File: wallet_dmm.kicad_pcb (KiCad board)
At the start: 2 copper layers, 86 x 53 mm, 26 parts, among them J1 Conn_01x04, J2 Conn_01x02, Q1 T2N7002BK_LM, Q2 T2N7002BK_LM, SW1 RESET_BUTTON, SW2 BUTTON0, SW3 BUTTON1, SW4 BUTTON2, U1 STM32L051K8Tx, U2 TLC555xD, U3 MCP9700-E/TO

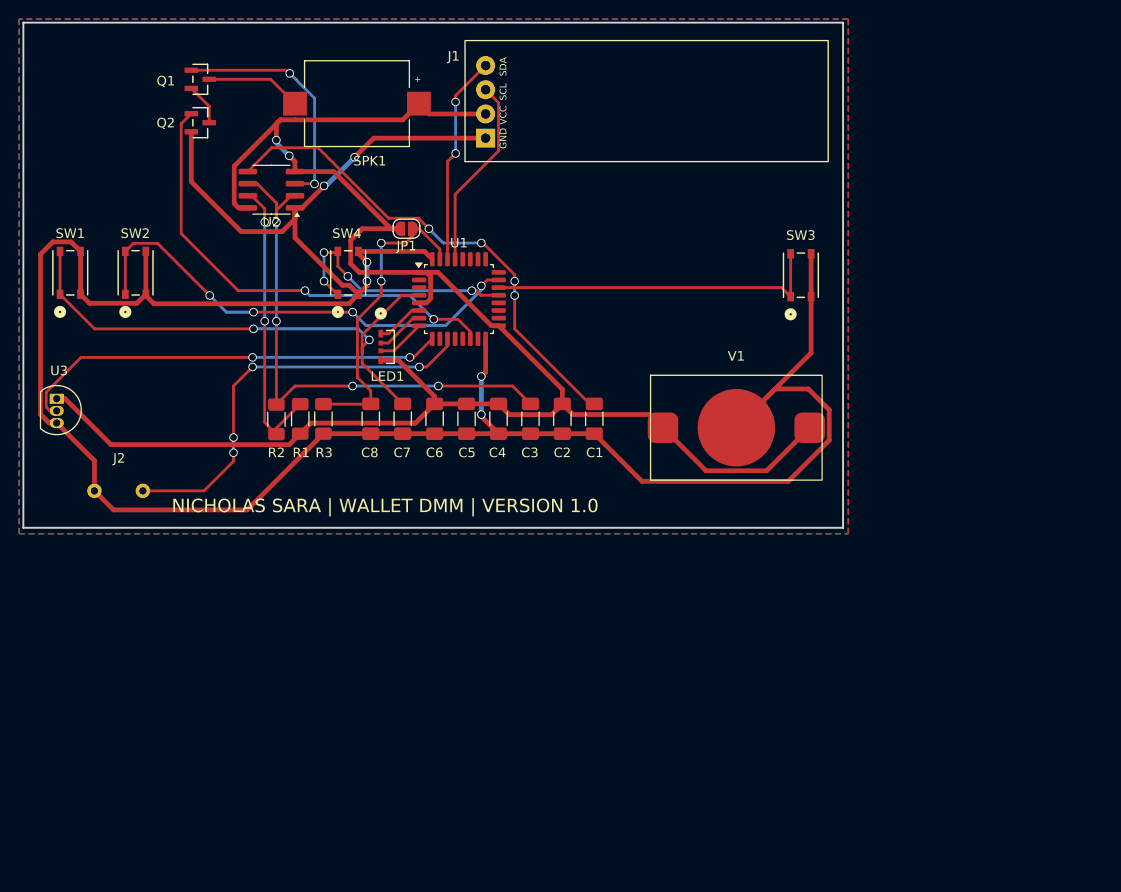
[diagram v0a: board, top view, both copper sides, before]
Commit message: Revision 2
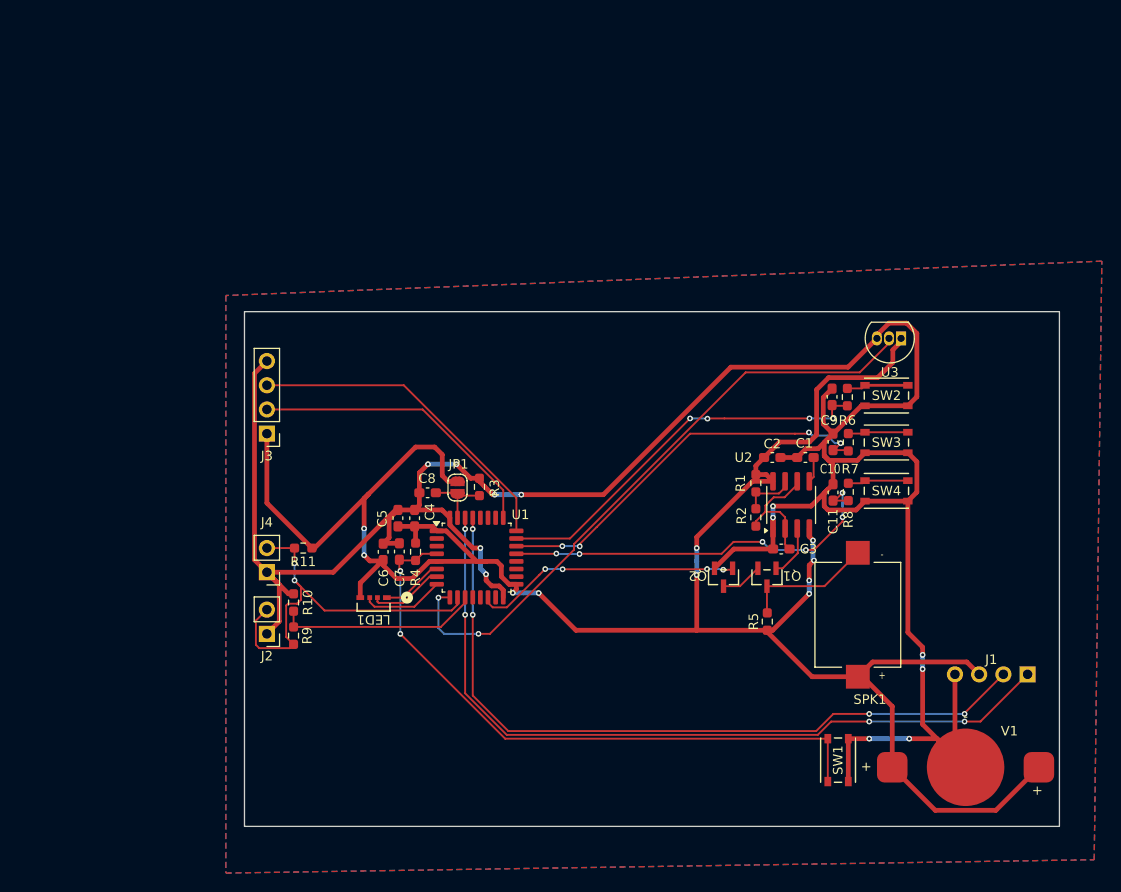
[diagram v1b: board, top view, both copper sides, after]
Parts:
- added C10: 100nF, Capacitor_SMD:C_0603_1608Metric_Pad1.08x0.95mm_HandSolder, F.Cu at (155.4, 72.9)
- added C11: 100nF, Capacitor_SMD:C_0603_1608Metric_Pad1.08x0.95mm_HandSolder, F.Cu at (155.4, 78.2)
- added C9: 100nF, Capacitor_SMD:C_0603_1608Metric_Pad1.08x0.95mm_HandSolder, F.Cu at (155.3, 68.1)
- added J3: Conn_01x04, Connector_PinHeader_2.54mm:PinHeader_1x04_P2.54mm_Vertical, F.Cu at (96.0, 72.0)
- added J4: Voltmeter, Connector_PinHeader_2.54mm:PinHeader_1x02_P2.54mm_Vertical, F.Cu at (96.0, 86.5)
- added R10: 1M, Resistor_SMD:R_0603_1608Metric_Pad0.98x0.95mm_HandSolder, F.Cu at (98.8, 89.7)
- added R11: 1M, Resistor_SMD:R_0603_1608Metric_Pad0.98x0.95mm_HandSolder, F.Cu at (99.8, 84.0)
- added R4: 10k, Resistor_SMD:R_0603_1608Metric_Pad0.98x0.95mm_HandSolder, F.Cu at (111.6, 84.4)
- added R5: 100, Resistor_SMD:R_0603_1608Metric_Pad0.98x0.95mm_HandSolder, F.Cu at (148.5, 91.7)
- added R6: 4.7k, Resistor_SMD:R_0603_1608Metric_Pad0.98x0.95mm_HandSolder, F.Cu at (156.9, 68.2)
- added R7: 4.7k, Resistor_SMD:R_0603_1608Metric_Pad0.98x0.95mm_HandSolder, F.Cu at (157.0, 72.9)
- added R8: 4.7k, Resistor_SMD:R_0603_1608Metric_Pad0.98x0.95mm_HandSolder, F.Cu at (157.0, 78.1)
- added R9: 10M, Resistor_SMD:R_0603_1608Metric_Pad0.98x0.95mm_HandSolder, F.Cu at (98.8, 93.2)
- C1, C2, C3, C4, C5, C6, C7, C8: footprint Capacitor_SMD:C_1206_3216Metric_Pad1.33x1.80mm_HandSolder -> Capacitor_SMD:C_0603_1608Metric_Pad1.08x0.95mm_HandSolder
- J1: footprint project_specific_footprints:OLED_Header -> custom:OLED_Header
- J2: value Conn_01x02 -> Voltmeter; footprint project_specific_footprints:ADC_Connector -> Connector_PinHeader_2.54mm:PinHeader_1x02_P2.54mm_Vertical
- LED1: footprint project_specific_footprints:QBLP615-RGB-3053_QTB -> project:QBLP615-RGB-3053_QTB
- Q1, Q2: footprint project_specific_footprints:T2N7002BK -> project:T2N7002BK
- R1, R2: footprint Resistor_SMD:R_1206_3216Metric_Pad1.30x1.75mm_HandSolder -> Resistor_SMD:R_0603_1608Metric_Pad0.98x0.95mm_HandSolder
- R3: value 1kR -> 10k; footprint Resistor_SMD:R_1206_3216Metric_Pad1.30x1.75mm_HandSolder -> Resistor_SMD:R_0603_1608Metric_Pad0.98x0.95mm_HandSolder
- SPK1: footprint project_specific_footprints:XDCR_CPT-1117-83-SMT-TR -> project:XDCR_CPT-1117-83-SMT-TR
- SW1, SW2, SW3, SW4: footprint project_specific_footprints:SW4_PTS815 SJM 250 SMTR LFS_CNK -> project:SW4_PTS815 SJM 250 SMTR LFS_CNK
- V1: footprint project_specific_footprints:BK-870_CR1025_Holder -> custom:BK-870-TR
- moved SW1 95.4 mm to (155.9, 106.3)
- moved U3 88.8 mm to (162.5, 62.0), turned to 180 degrees
- moved J1 85.0 mm to (172.0, 97.2)
- moved SW2 79.8 mm to (161.0, 68.0), turned to 0 degrees
- moved Q1 79.1 mm to (148.5, 87.1), turned to 180 degrees
- moved SPK1 75.1 mm to (158.0, 91.0), turned to 180 degrees
- moved Q2 72.7 mm to (143.9, 87.1), turned to 180 degrees
- moved U2 63.8 mm to (151.0, 79.5), turned to 90 degrees
- moved SW4 60.9 mm to (161.0, 78.0), turned to 0 degrees
- moved R2 51.3 mm to (147.3, 80.8), turned to -90 degrees
- moved R1 48.3 mm to (147.3, 77.2), turned to -90 degrees
- moved V1 43.0 mm to (169.3, 107.0)
- moved C3 29.7 mm to (150.0, 84.1), turned to 180 degrees
- moved JP1 27.7 mm to (116.0, 77.7), turned to 90 degrees
- moved U1 27.2 mm to (118.0, 85.0)
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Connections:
- net BOOT0 renamed /BOOT0
- net I2C1_SCL renamed /I2C1_SCL
- net I2C1_SDA renamed /I2C1_SDA
- net LED_BLUE renamed /LED_BLUE
- net LED_GREEN renamed /LED_GREEN
- net LED_RED renamed /LED_RED
- net NRST renamed /NRST
- net OSC_OUT renamed /PIEZO_OUT
- net PIEZO_EN renamed /PIEZO_EN
- net TEMP_ADC renamed /TEMP_ADC
- net VDD renamed VCC
- J2 pad 1: ADC -> GND
- J2 pad 2: GND -> /CONTINUITY
- SW2 pad 1: BUTTON0 -> Net-(R6-Pad1)
- SW2 pad 2: BUTTON0 -> Net-(R6-Pad1)
- SW3 pad 1: BUTTON1 -> Net-(R7-Pad1)
- SW3 pad 2: BUTTON1 -> Net-(R7-Pad1)
- SW4 pad 1: BUTTON2 -> Net-(R8-Pad1)
- SW4 pad 2: BUTTON2 -> Net-(R8-Pad1)
- U1 pad 10: unconnected-(U1-PA4-Pad10) -> /CONTINUITY
- U1 pad 11: ADC -> /ADC
- U1 pad 21: BUTTON2 -> /BUTTON2
- U1 pad 22: BUTTON1 -> /BUTTON1
- U1 pad 23: BUTTON0 -> /BUTTON0
- U1 pad 24: unconnected-(U1-PA14-Pad24) -> /SWCLK
- U1 pad 25: unconnected-(U1-PA15-Pad25) -> /SWDIO
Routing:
- net /I2C1_SDA: track 22.0 -> 81.9 mm, vias 2 -> 4
- net /I2C1_SCL: track 20.2 -> 78.4 mm, vias 0 -> 4
- net BUTTON0: track 49.8 -> 0.00 mm, vias 4 -> 0
- net Net-(U2-CV): track 51.8 -> 2.69 mm, vias 4 -> 0
- net Net-(U2-THR): track 57.0 -> 13.0 mm, vias 4 -> 0
- net ADC: track 43.6 -> 0.00 mm, vias 4 -> 0
- net /BUTTON2: track 0.00 -> 43.0 mm, vias 0 -> 6
- net /CONTINUITY: track 0.00 -> 42.6 mm, vias 0 -> 2
- net /BUTTON1: track 0.00 -> 42.3 mm, vias 0 -> 4
- net /BUTTON0: track 0.00 -> 41.5 mm, vias 0 -> 4
- net BUTTON1: track 35.5 -> 0.00 mm
- net /SWCLK: track 0.00 -> 34.5 mm
- net VCC: track 194.0 -> 226.6 mm, vias 2 -> 10
- net /SWDIO: track 0.00 -> 31.2 mm
- net BUTTON2: track 26.2 -> 0.00 mm, vias 4 -> 0
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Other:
- board size 86 x 53 mm -> 85.5 x 54 mm
- board text removed: "NICHOLAS SARA | WALLET DMM | VERSION 1.0"
